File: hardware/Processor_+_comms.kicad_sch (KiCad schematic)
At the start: 50 parts, among them J1 53261-0471, U11 ATXMEGA256A3U-MH, U12 NTS0104, U13 CYPD3177, U14 TC1015-3.3VCT713

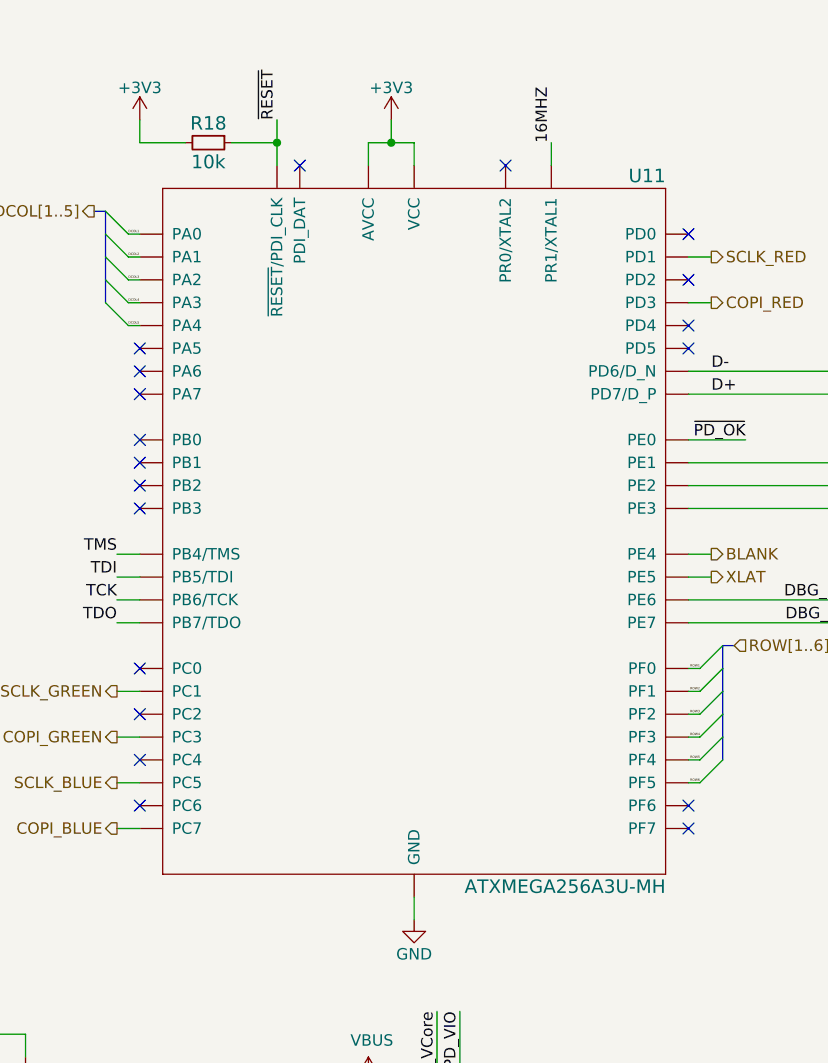
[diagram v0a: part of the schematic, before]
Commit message: Further updates to the board files
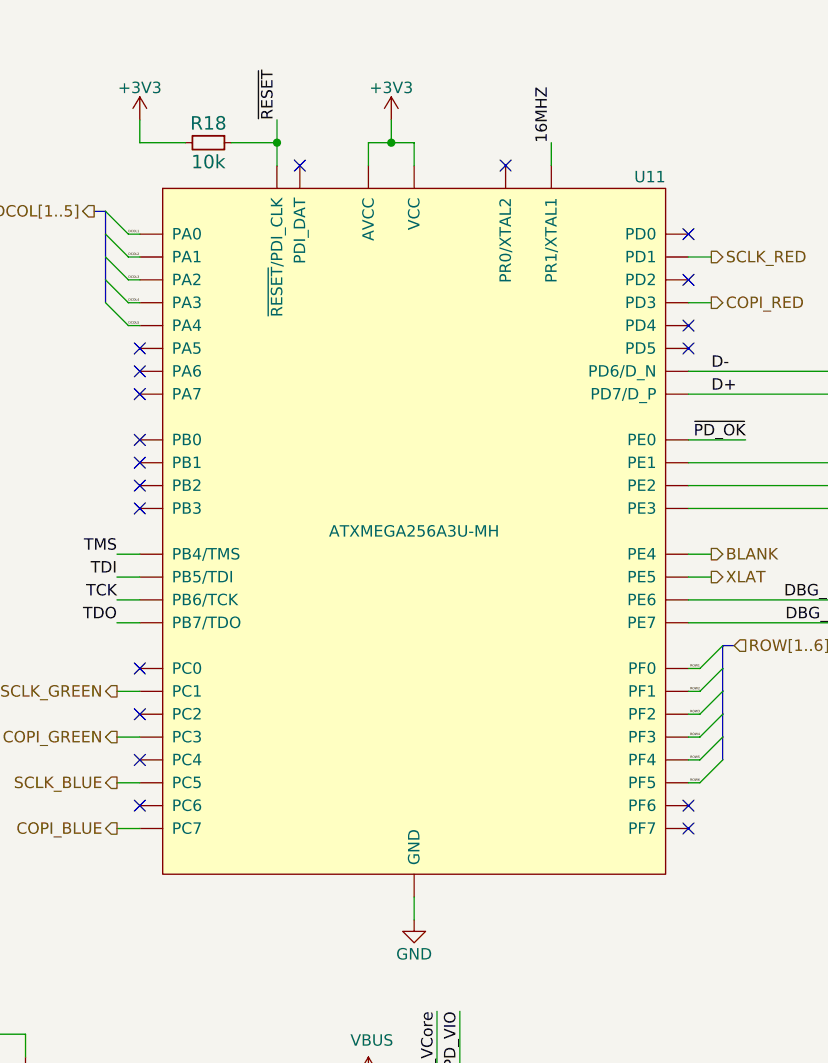
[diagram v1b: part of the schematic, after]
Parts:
- U11: symbol MXKeyboard-eagle-import:ATXMEGA256A3U-MH -> DX-MON:ATXMEGA256A3U-MH
- U12: symbol MXKeyboard-eagle-import:NTS0104 -> DX-MON:NTS0104
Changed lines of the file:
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@@
     (pin "9")
   )
-  (symbol (lib_id "MXKeyboard-eagle-import:ATXMEGA256A3U-MH") (at 144.78 147.32 0) (unit 1)
-    (in_bom yes) (on_board yes)
-    (property "Reference" "U11" (id 0) (at 172.72 108.712 0)
-      (effects (font (size 1.4986 1.4986)) (justify right bottom))
-    )
-    (property "Value" "ATXMEGA256A3U-MH" (id 1) (at 172.72 185.928 0)
-      (effects (font (size 1.4986 1.4986)) (justify right top))
-    )
+  (symbol (lib_id "DX-MON:ATXMEGA256A3U-MH") (at 144.78 147.32 0) (unit 1)
+    (in_bom yes) (on_board yes)
+    (property "Reference" "U11" (id 0) (at 172.72 107.95 0)
+      (effects (font (size 1.27 1.27)) (justify right))
+    )
+    (property "Value" "ATXMEGA256A3U-MH" (id 1) (at 144.78 147.32 0))
     (property "Footprint" "rhais_package-qfn:QFN-64-1EP_9x9mm_P0.5mm_EP7.5x7.5mm" (id 2) (at 144.78 147.32 0)
       (effects (font (size 1.27 1.27)) hide)
@@
     (pin "5")
   )
-  (symbol (lib_id "MXKeyboard-eagle-import:NTS0104") (at 317.5 165.1 0) (unit 1)
+  (symbol (lib_id "DX-MON:NTS0104") (at 317.5 165.1 0) (unit 1)
     (in_bom yes) (on_board yes)
     (property "Reference" "U12" (id 0) (at 327.66 179.07 0)
